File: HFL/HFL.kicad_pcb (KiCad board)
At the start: 2 copper layers, 62.6 x 37.6 mm, 82 parts, among them J1 STS_IO, J2 Conn_01x06_Male, J3 PWR, Q1 2N7002, Q2 MCT06P10-TP, Q3 2N7002, SW1 RST, SW2 BYPASS, U1 74LS32, U2 74LS08, U3 MCP6004, U4 LM1117-5.0, U5 4044, U6 NE555, U7 LTV-817S

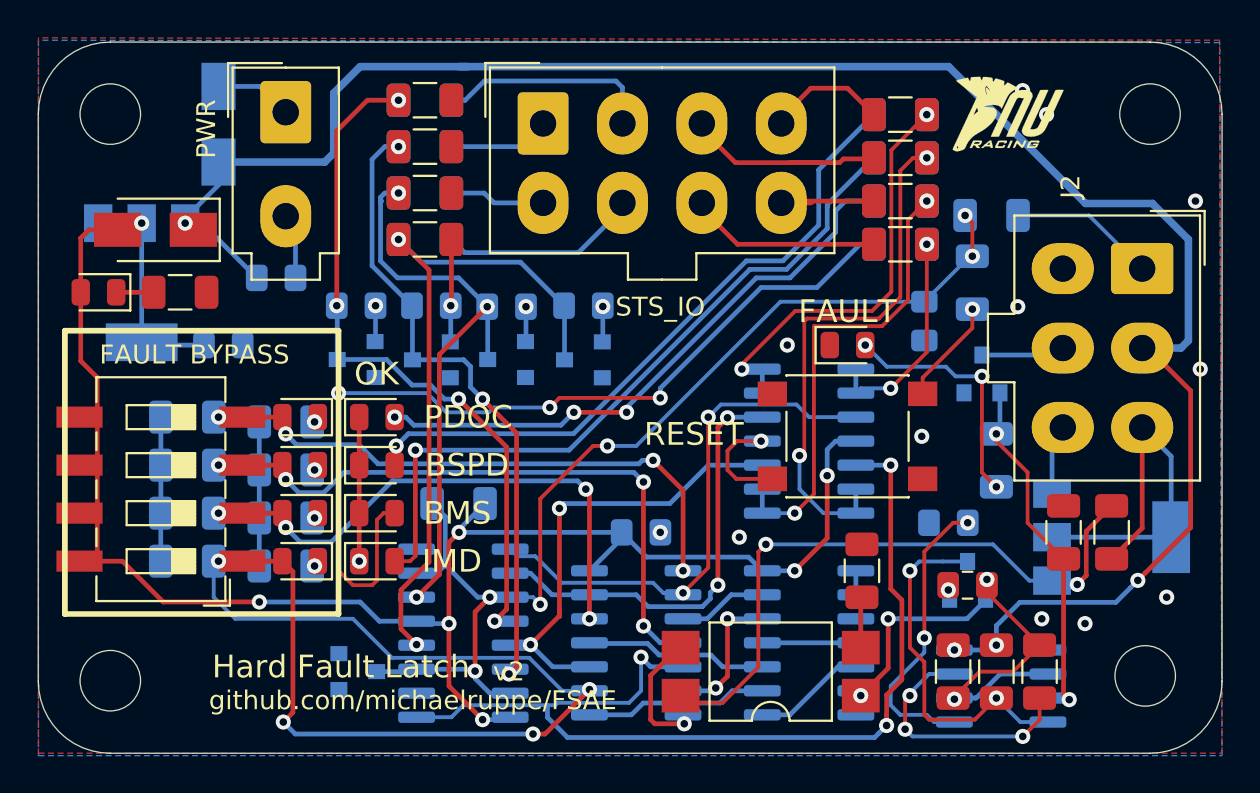
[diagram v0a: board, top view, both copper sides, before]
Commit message: Lock down before branch for projects
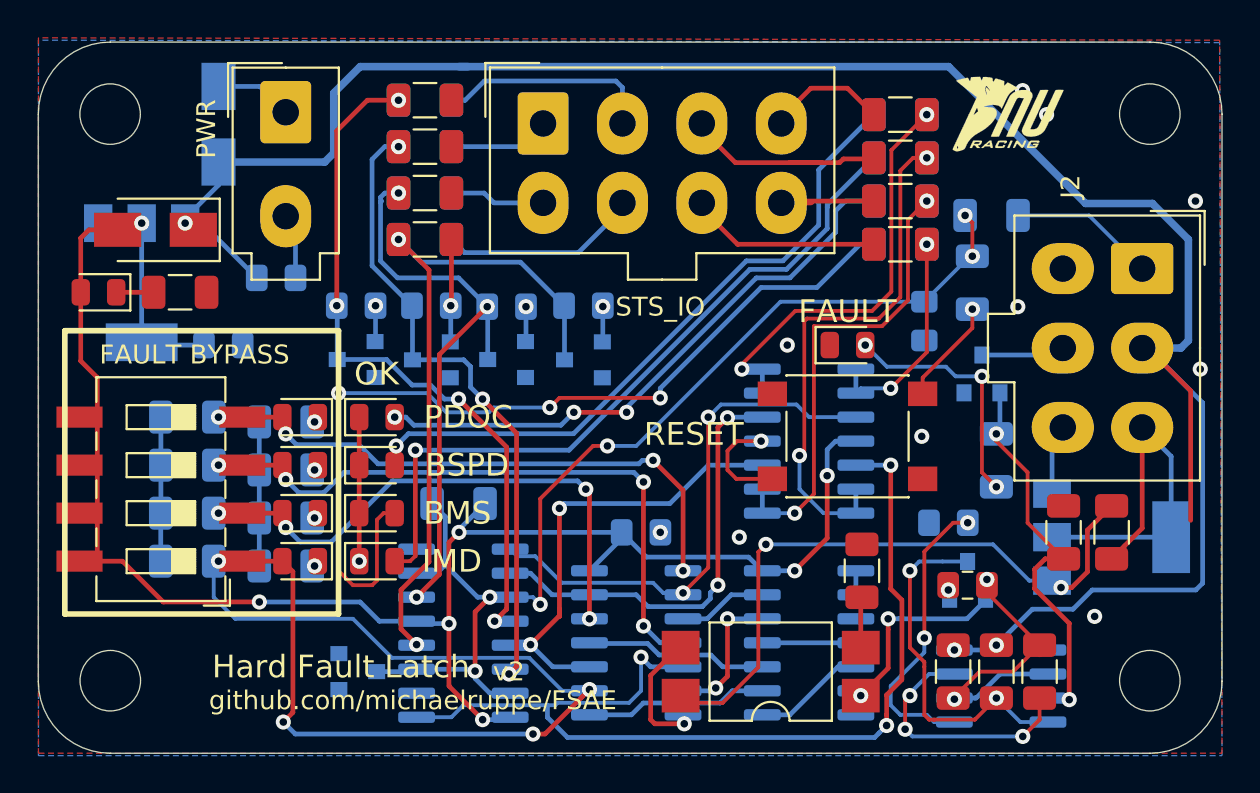
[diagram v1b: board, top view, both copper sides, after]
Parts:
- moved REF** 0.35 mm to (135.0, 79.5)
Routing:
- net +12V: track 103.0 -> 115.4 mm, vias 4 -> 3
- net Net-(Q3-Pad1): track 19.1 -> 20.9 mm
- net GND: vias 20 -> 18
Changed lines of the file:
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@@
     (thickness 1.6)
     (drawings 24)
-    (tracks 655)
+    (tracks 658)
     (zones 0)
     (modules 82)
@@
     (pad_to_mask_clearance 0.051)
     (solder_mask_min_width 0.25)
-    (aux_axis_origin 0 0)
+    (aux_axis_origin 80.01 79.53)
     (grid_origin 80.01 79.53)
     (visible_elements 7FFFFFFF)
@@
     (add_net SHTDN_OUT)
   )
-  (module MountingHole:MountingHole_3.2mm_M3 (layer F.Cu)
-    (at 134.756 79.248)
+  (module MountingHole:MountingHole_3.2mm_M3 locked (layer F.Cu)
+    (at 135 79.502)
     (descr "Mounting Hole 3.2mm, no annular, M3")
     (tags "mounting hole 3.2mm no annular m3")
@@
   )
   (module MountingHole:MountingHole_3.2mm_M3 locked (layer F.Cu)
-    (at 135.01 49.53)
+    (at 135 49.53)
     (descr "Mounting Hole 3.2mm, no annular, M3")
     (tags "mounting hole 3.2mm no annular m3")
@@
   )
   (module MountingHole:MountingHole_3.2mm_M3 locked (layer F.Cu)
-    (at 80.01 49.53)
+    (at 80 49.53)
     (descr "Mounting Hole 3.2mm, no annular, M3")
     (tags "mounting hole 3.2mm no annular m3")
@@
   (via (at 128.016 59.718) (size 0.8) (drill 0.4) (layers F.Cu B.Cu) (net 1))
   (via (at 115.824 61.75) (size 0.8) (drill 0.4) (layers F.Cu B.Cu) (net 1))
-  (via (at 131.572 76.482) (size 0.8) (drill 0.4) (layers F.Cu B.Cu) (net 1))
   (segment (start 115.033 68.826) (end 113.13 68.826) (width 0.2032) (layer F.Cu) (net 1) (status 10))
   (via (at 113.284 71.91) (size 0.8) (drill 0.4) (layers F.Cu B.Cu) (net 1))
-  (via (at 129.286 76.228) (size 0.8) (drill 0.4) (layers F.Cu B.Cu) (net 1))
-  (via (at 135.89 75.085) (size 0.8) (drill 0.4) (layers F.Cu B.Cu) (net 1))
+  (via (at 132.08 76.101) (size 0.8) (drill 0.4) (layers F.Cu B.Cu) (net 1))
   (segment (start 80.3215 58.956) (end 82.302 58.956) (width 0.25) (layer F.Cu) (net 2) (status 30))
   (via (at 90.814 73.434) (size 0.8) (drill 0.4) (layers F.Cu B.Cu) (net 3) (status 30))
@@
   (segment (start 124.661 77.879) (end 126.625 77.879) (width 0.25) (layer B.Cu) (net 4) (status 10))
   (via (at 124.661 77.879) (size 0.8) (drill 0.4) (layers F.Cu B.Cu) (net 4) (status 30))
-  (segment (start 134.765999 73.796001) (end 134.366 74.196) (width 0.25) (layer F.Cu) (net 4))
-  (segment (start 134.596 61.904) (end 134.896 61.904) (width 0.25) (layer F.Cu) (net 4))
+  (segment (start 137.16 64.168) (end 137.16 71.021) (width 0.25) (layer F.Cu) (net 4))
   (segment (start 134.896 61.904) (end 137.16 64.168) (width 0.25) (layer F.Cu) (net 4))
-  (segment (start 137.16 64.168) (end 137.16 71.402) (width 0.25) (layer F.Cu) (net 4))
-  (segment (start 137.16 71.402) (end 134.765999 73.796001) (width 0.25) (layer F.Cu) (net 4))
-  (via (at 134.366 74.196) (size 0.8) (drill 0.4) (layers F.Cu B.Cu) (net 4))
-  (segment (start 133.966001 74.595999) (end 134.366 74.196) (width 0.25) (layer B.Cu) (net 4))
-  (segment (start 133.204001 75.357999) (end 133.966001 74.595999) (width 0.25) (layer B.Cu) (net 4))
-  (segment (start 128.124001 75.357999) (end 133.204001 75.357999) (width 0.25) (layer B.Cu) (net 4))
-  (segment (start 126.882 77.622) (end 126.882 76.6) (width 0.25) (layer B.Cu) (net 4))
-  (segment (start 126.882 76.6) (end 128.124001 75.357999) (width 0.25) (layer B.Cu) (net 4))
+  (segment (start 134.596 61.904) (end 134.896 61.904) (width 0.25) (layer F.Cu) (net 4))
+  (segment (start 137.795 64.803) (end 134.896 61.904) (width 0.25) (layer B.Cu) (net 4))
+  (segment (start 128.784 75.72) (end 130.937 75.72) (width 0.25) (layer B.Cu) (net 4))
+  (segment (start 126.882 77.622) (end 128.784 75.72) (width 0.25) (layer B.Cu) (net 4))
+  (segment (start 134.896 61.904) (end 134.596 61.904) (width 0.25) (layer B.Cu) (net 4))
+  (segment (start 130.937 75.72) (end 131.953 74.704) (width 0.25) (layer B.Cu) (net 4))
+  (segment (start 131.953 74.704) (end 137.432999 74.704) (width 0.25) (layer B.Cu) (net 4))
+  (segment (start 137.432999 74.704) (end 137.795 74.341999) (width 0.25) (layer B.Cu) (net 4))
+  (segment (start 137.795 74.341999) (end 137.795 64.803) (width 0.25) (layer B.Cu) (net 4))
   (via (at 95.256 56.162) (size 0.8) (drill 0.4) (layers F.Cu B.Cu) (net 5) (status 30))
   (segment (start 104.038 59.689666) (end 104.013 59.664666) (width 0.25) (layer B.Cu) (net 5) (status 30))
@@
   (via (at 90.814 68.354) (size 0.8) (drill 0.4) (layers F.Cu B.Cu) (net 39) (status 30))
   (via (at 90.814 65.814) (size 0.8) (drill 0.4) (layers F.Cu B.Cu) (net 40) (status 30))
-  (via (at 131.16301 74.412988) (size 0.8) (drill 0.4) (layers F.Cu B.Cu) (net 41))
-  (segment (start 132.978 70.256) (end 131.63801 71.59599) (width 0.25) (layer F.Cu) (net 41) (status 10))
-  (segment (start 131.63801 71.59599) (end 131.63801 73.937988) (width 0.25) (layer F.Cu) (net 41))
-  (segment (start 131.63801 73.937988) (end 131.16301 74.412988) (width 0.25) (layer F.Cu) (net 41))
   (segment (start 128.6248 74.21) (end 126.7058 72.291) (width 0.2032) (layer B.Cu) (net 41))
   (segment (start 129.828 74.21) (end 128.6248 74.21) (width 0.2032) (layer B.Cu) (net 41) (status 10))
@@
   (segment (start 114.69 72.291) (end 114.290001 72.690999) (width 0.2032) (layer F.Cu) (net 41))
   (segment (start 114.290001 72.690999) (end 114.290001 78.786999) (width 0.2032) (layer F.Cu) (net 41))
-  (segment (start 130.960022 74.21) (end 131.16301 74.412988) (width 0.2032) (layer B.Cu) (net 41))
-  (segment (start 129.828 74.21) (end 130.960022 74.21) (width 0.2032) (layer B.Cu) (net 41) (status 10))
+  (segment (start 129.828 74.21) (end 129.860999 74.177001) (width 0.2032) (layer B.Cu) (net 41))
+  (segment (start 132.978 70.256) (end 131.699 71.535) (width 0.25) (layer F.Cu) (net 41))
+  (segment (start 129.860999 74.177001) (end 129.902001 74.177001) (width 0.2032) (layer B.Cu) (net 41))
+  (segment (start 129.902001 74.177001) (end 130.302 74.577) (width 0.2032) (layer B.Cu) (net 41))
+  (segment (start 130.867685 74.577) (end 130.302 74.577) (width 0.25) (layer F.Cu) (net 41))
+  (segment (start 131.699 73.745685) (end 130.867685 74.577) (width 0.25) (layer F.Cu) (net 41))
+  (via (at 130.302 74.577) (size 0.8) (drill 0.4) (layers F.Cu B.Cu) (net 41))
+  (segment (start 131.699 71.535) (end 131.699 73.745685) (width 0.25) (layer F.Cu) (net 41))
   (segment (start 127.07 66.258) (end 126.882 66.446) (width 0.25) (layer B.Cu) (net 42) (status 30))
   (segment (start 127.07 64.274) (end 127.07 66.258) (width 0.25) (layer B.Cu) (net 42) (status 30))
@@
   (segment (start 128.533 68.481) (end 126.882 66.83) (width 0.2032) (layer F.Cu) (net 42))
   (segment (start 126.882 66.83) (end 126.882 66.446) (width 0.2032) (layer F.Cu) (net 42))
-  (segment (start 130.438 73.056) (end 130.438 80.20591) (width 0.25) (layer F.Cu) (net 42) (status 10))
   (via (at 130.736824 80.504734) (size 0.8) (drill 0.4) (layers F.Cu B.Cu) (net 42))
-  (segment (start 130.438 80.20591) (end 130.736824 80.504734) (width 0.25) (layer F.Cu) (net 42))
   (segment (start 129.696734 80.504734) (end 129.611 80.419) (width 0.25) (layer B.Cu) (net 42) (status 30))
   (segment (start 130.736824 80.504734) (end 129.696734 80.504734) (width 0.25) (layer B.Cu) (net 42) (status 20))
+  (segment (start 130.736824 80.504734) (end 130.736824 76.465826) (width 0.25) (layer F.Cu) (net 42))
+  (segment (start 128.905 73.614) (end 129.463 73.056) (width 0.25) (layer F.Cu) (net 42))
+  (segment (start 129.463 73.056) (end 130.438 73.056) (width 0.25) (layer F.Cu) (net 42))
+  (segment (start 128.905 74.634002) (end 128.905 73.614) (width 0.25) (layer F.Cu) (net 42))
+  (segment (start 130.736824 76.465826) (end 128.905 74.634002) (width 0.25) (layer F.Cu) (net 42))
   (via (at 125.612 59.848) (size 0.8) (drill 0.4) (layers F.Cu B.Cu) (net 43) (status 30))
   (segment (start 125.612 60.8438) (end 125.612 59.848) (width 0.2032) (layer F.Cu) (net 43))
